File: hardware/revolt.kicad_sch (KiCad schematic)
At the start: 22 parts, among them M1 Motor_DC, M2 Motor_DC, M3 Motor_DC, M4 Motor_DC, SW1 SW_Push, U1 HC-06, U2 PCF8574, U3 ADXL345, U4 L293, U5 USPRO_LM393, U6 HC-SRO4, U7 BW-3SJH-25A

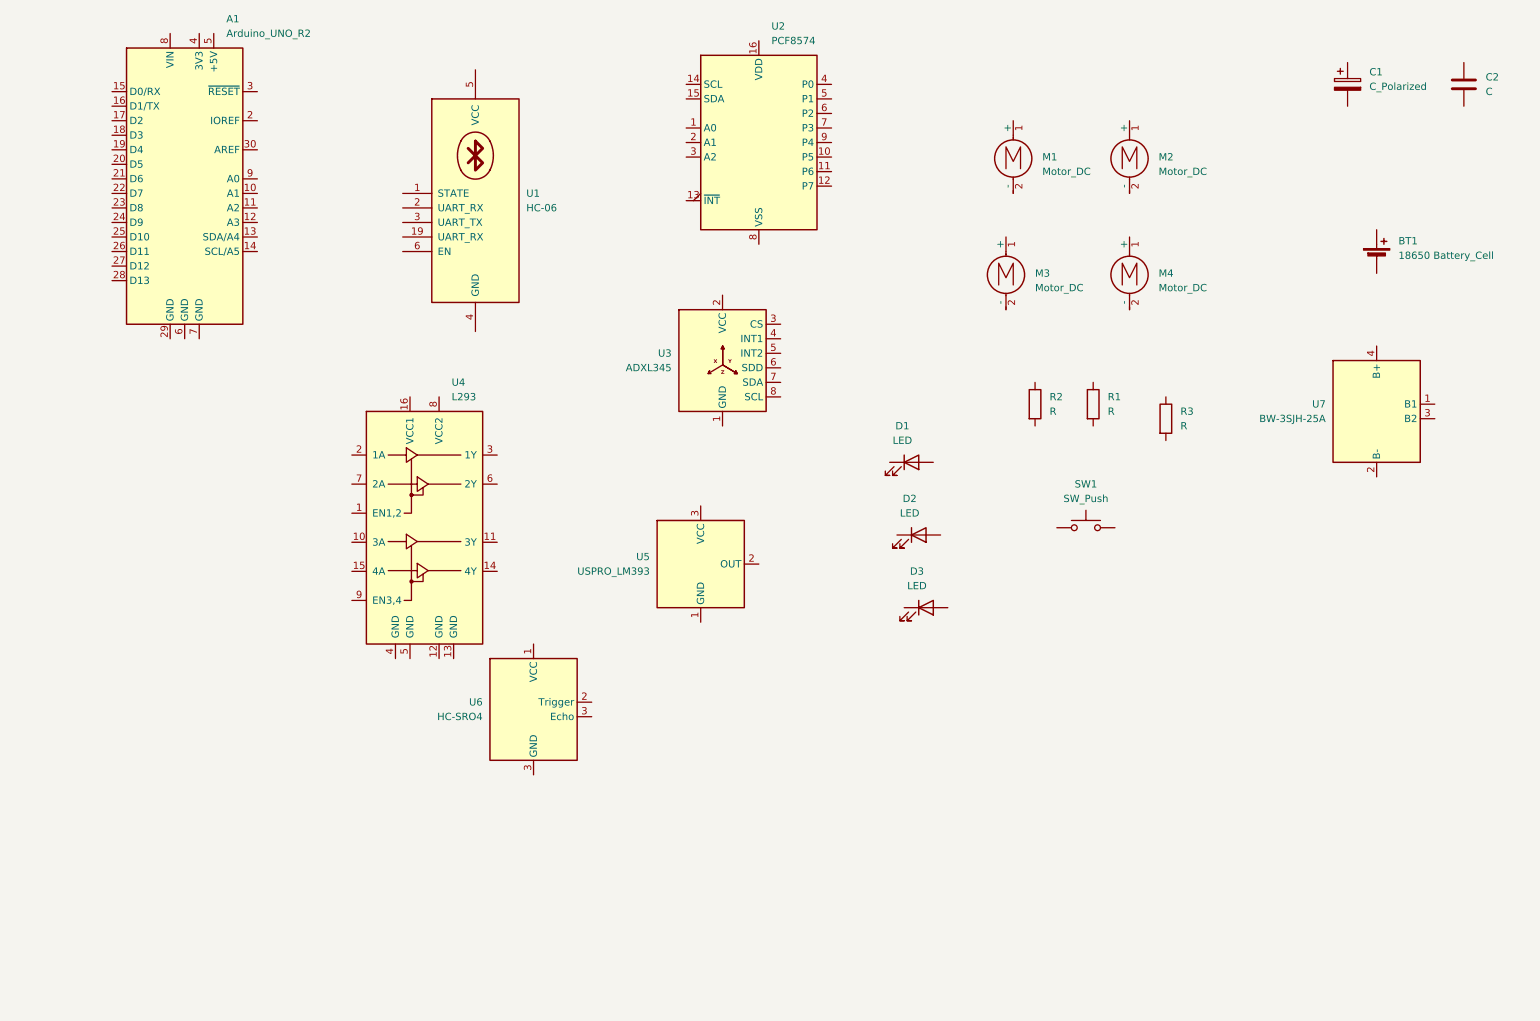
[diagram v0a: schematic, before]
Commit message: finish diagram
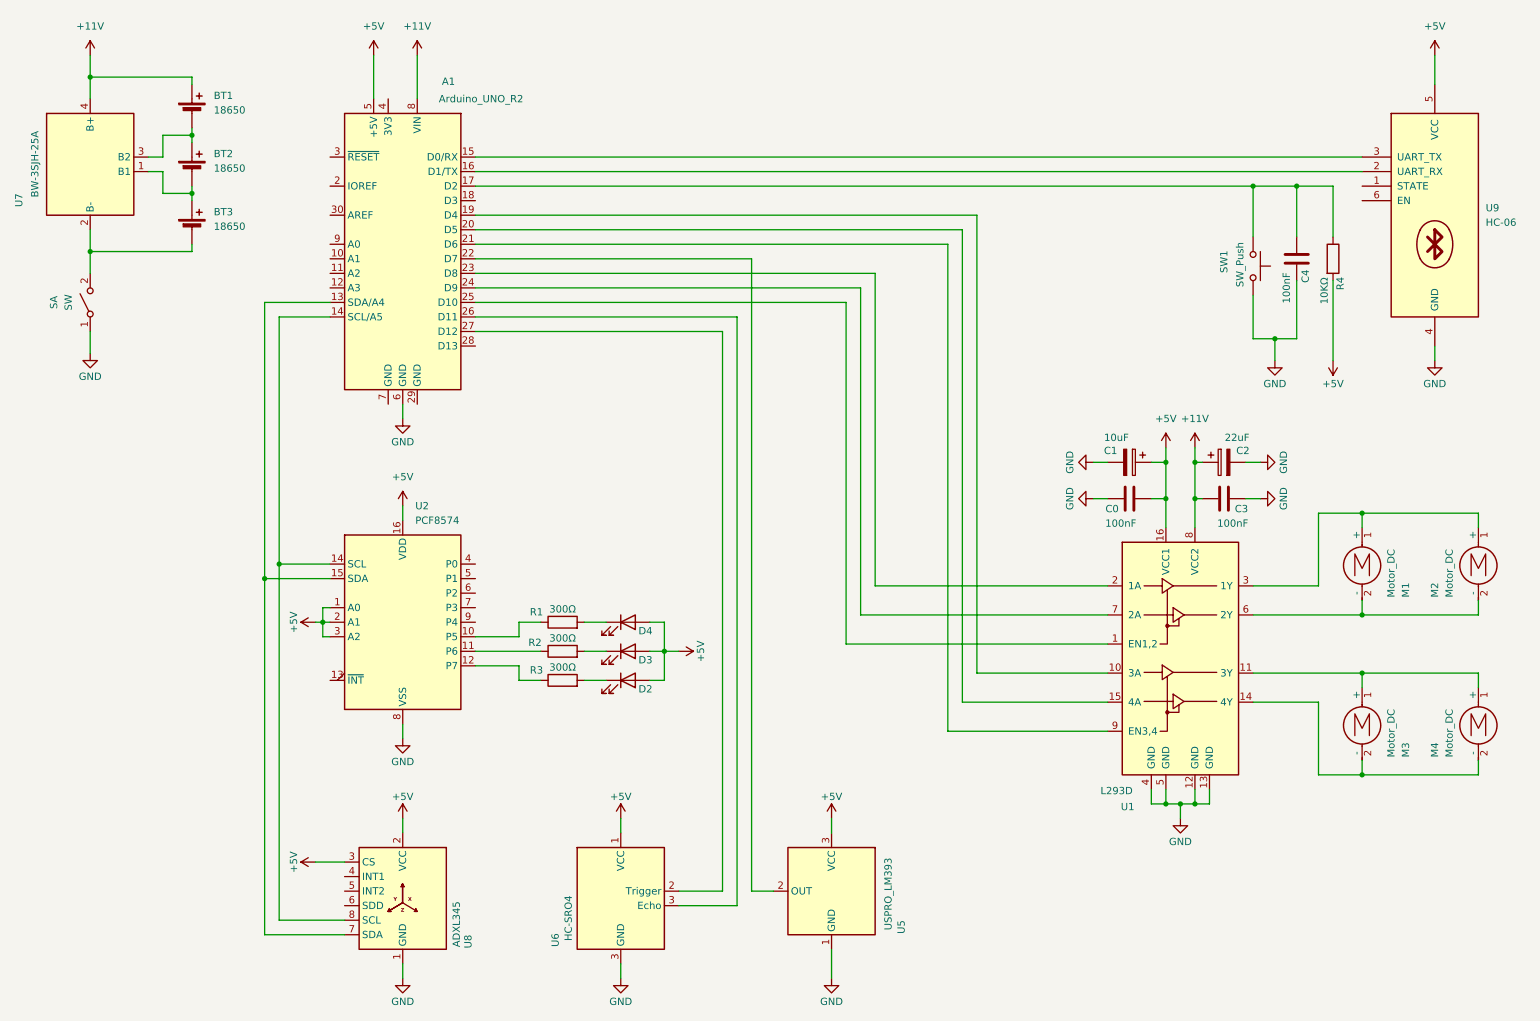
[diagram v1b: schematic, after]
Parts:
- removed D1: LED, symbol Device:LED
- removed U1: HC-06, symbol elements:HC-06
- removed U3: ADXL345, symbol elements:ADXL345
- removed U4: L293, Package_DIP:DIP-16_W7.62mm, symbol Driver_Motor:L293
- added BT2, BT3: 18650, symbol Device:Battery_Cell
- added C2: 22uF, symbol Device:C_Polarized
- added C3, C4: 100nF, symbol Device:C
- added D4: LED, symbol Device:LED
- added R4: 10KΩ, symbol Device:R
- added S: SW, symbol Switch:SW_DPST_x2
- added U1: L293D, Package_DIP:DIP-16_W7.62mm, symbol Driver_Motor:L293D
- added U8: ADXL345, symbol elements:ADXL345
- added U9: HC-06, symbol elements:HC-06
- BT1: value 18650 Battery_Cell -> 18650
- C0: renamed from C2; value C -> 100nF
- C1: value C_Polarized -> 10uF
- R1, R2, R3: value R -> 300Ω
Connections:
- net GND: now reaches C0.1
- net GND: now also A1.6 (GND), C1.2, SW1.2, U2.8 (VSS), U5.1 (GND), U6.3 (GND), C2.2, C3.1, C4.2, S.1 (A), U1.12 (GND), U1.13 (GND), U1.4 (GND), U1.5 (GND), U8.1 (GND), U9.4 (GND)
- net +5V: now reaches C0.2
- net +5V: now also A1.5 (+5V), C1.1, D2.2 (A), D3.2 (A), U2.1 (A0), U2.16 (VDD), U2.2 (A1), U2.3 (A2), U5.3 (VCC), U6.1 (VCC), D4.2 (A), R4.2, U1.16 (VCC1), U8.2 (VCC), U8.3 (CS), U9.5 (VCC)
- net at R3.1: now also U2.12 (P7)
- net at R3.2: now also D2.1 (K)
- net at M4.1 (+): now also M3.1 (+), U1.11 (3Y)
- net at M4.2 (-): now also M3.2 (-), U1.14 (4Y)
- net at A1.13 (SDA/A4): now also U2.15 (SDA), U8.7 (SDA)
- net at A1.14 (SCL/A5): now also U2.14 (SCL), U8.8 (SCL)
- net at A1.15 (D0/RX): now also U9.3 (UART_TX)
- net at A1.16 (D1/TX): now also U9.2 (UART_RX)
- net at A1.17 (D2): now also SW1.1, C4.1, R4.1
- net at A1.19 (D4): now also U1.10 (3A)
- net at A1.20 (D5): now also U1.15 (4A)
- net at A1.21 (D6): now also U1.9 (EN3,4)
- net at A1.22 (D7): now also U5.2 (OUT)
- net at A1.23 (D8): now also U1.2 (1A)
- net at A1.24 (D9): now also U1.7 (2A)
- net at A1.25 (D10): now also U1.1 (EN1,2)
- net at A1.26 (D11): now also U6.3 (GND)
- net at A1.27 (D12): now also U6.2 (Trigger)
- net +11V: now reaches A1.8 (VIN)
- net +11V: now also BT1.1 (+), U7.4 (B+), C2.1, C3.2, U1.8 (VCC2)
- net at M2.1 (+): now also M1.1 (+), U1.3 (1Y)
- net at M2.2 (-): now also M1.2 (-), U1.6 (2Y)
- net at D3.1 (K): now also R2.2
- net at R1.1: now also U2.10 (P5)
- net at R1.2: now also D4.1 (K)
- net at U2.11 (P6): now also R2.1
- net at U7.1 (B1): now also BT2.2 (-), BT3.1 (+)
- net at U7.2 (B-): now also BT3.2 (-), S.2 (B)
- net at U7.3 (B2): now also BT1.2 (-), BT2.1 (+)
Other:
- moved on the sheet: A1, BT1, C0, C1, M1, M2, SW1, U2, U5, U6
